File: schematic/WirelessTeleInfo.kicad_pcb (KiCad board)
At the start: 2 copper layers, 25.4 x 26 mm, 9 parts, among them P2 TeleInfo, Q1 BS170, U1 LTV-814, U2 WeMos_mini

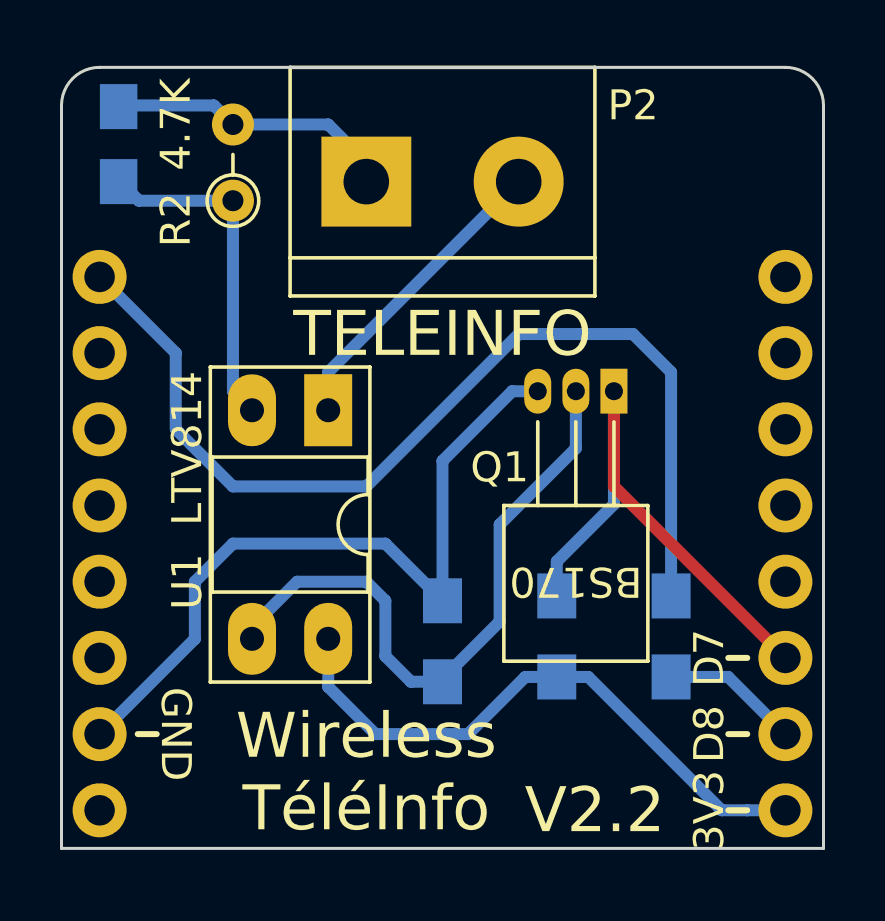
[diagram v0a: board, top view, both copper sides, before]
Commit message: Cleanup and update schematic to KiCAD 8
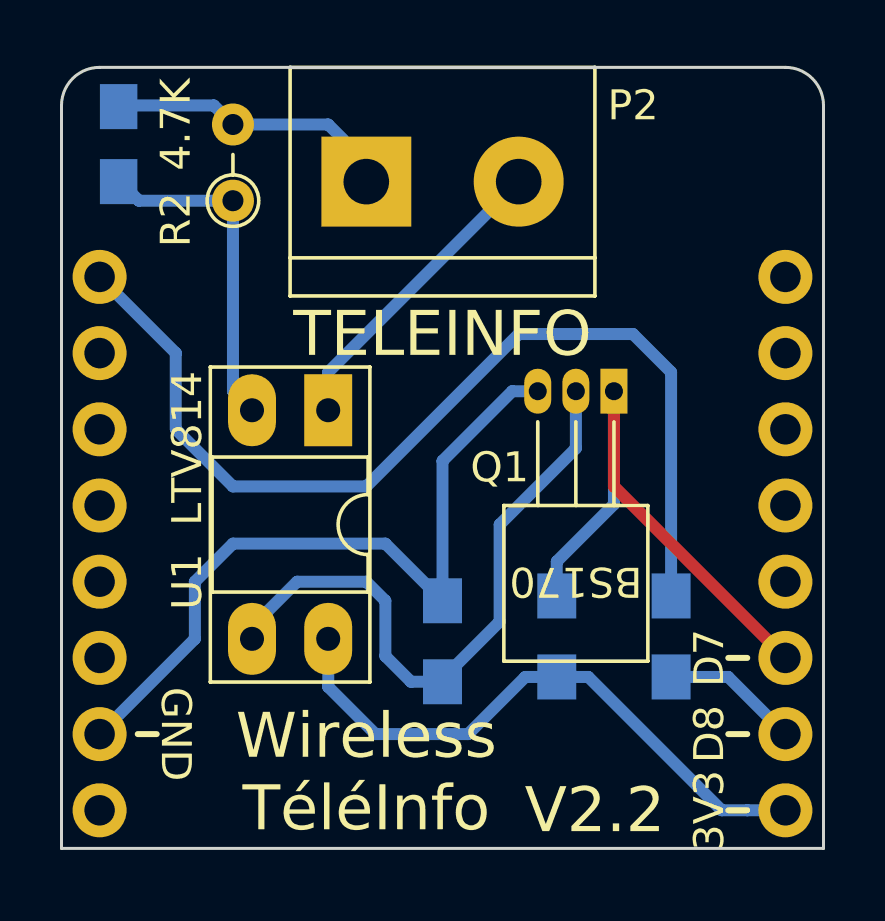
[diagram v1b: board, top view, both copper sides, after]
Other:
- net class Default removed
